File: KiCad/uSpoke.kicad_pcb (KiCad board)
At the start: 2 copper layers, 50 x 100 mm, 89 parts, among them J1 B2B-PH-K-S, J12 Amphenol 132289, J2 BAT+, J3 BAT-, J5 USB+, J6 USB-, J8 PLS-1x6, J9 PLS-1x3, Q1 AO3407A, Q2 AO3407A, Q3 AO3400, Q4 AO3400, Q5 AO3400, U2 TP4056, U4 LM3671MF-3.3, U6 STM32F103C8T6, X1 8MHz

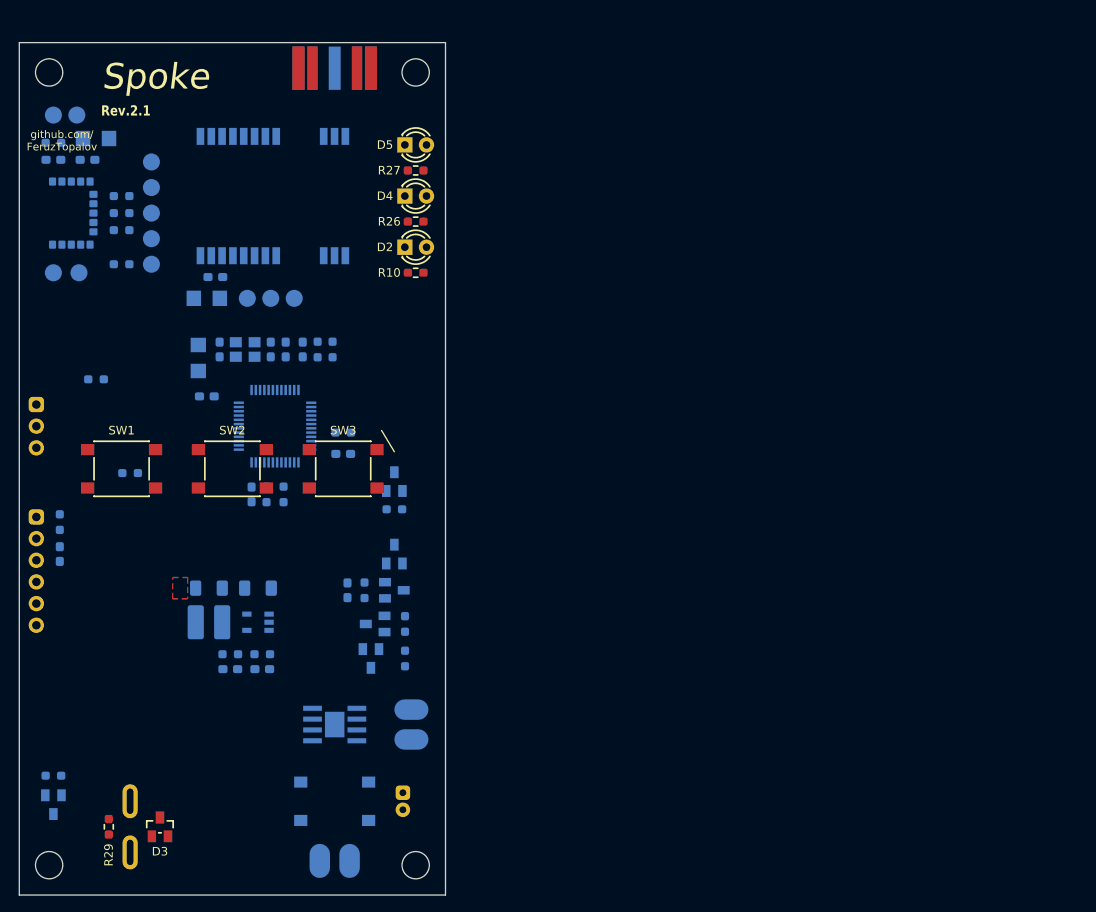
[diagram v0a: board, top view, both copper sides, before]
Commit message: Arrangement
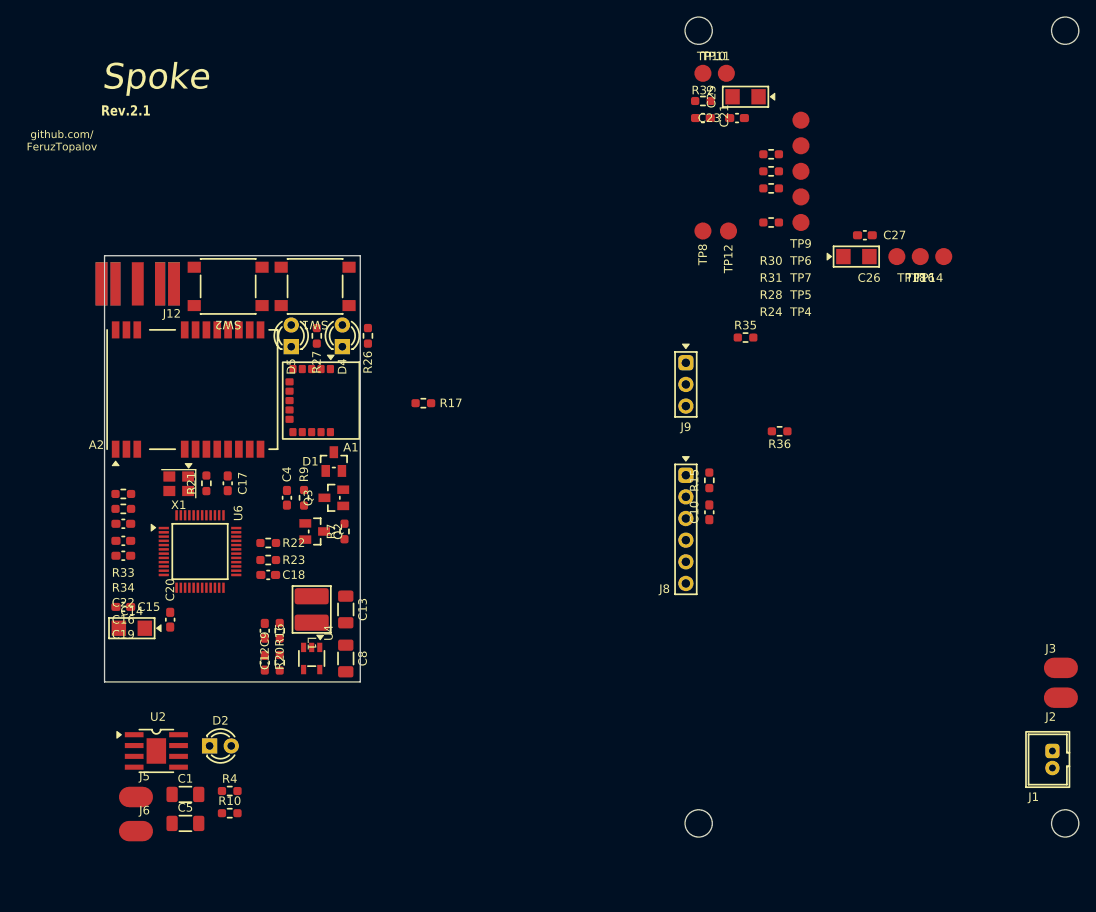
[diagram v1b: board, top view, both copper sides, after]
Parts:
- removed D3: BAT54C, Spoke:SOT-23
- removed LS1: Buzzer-Passive, Spoke:Buzzer
- removed Q1: AO3407A, Spoke:SOT-23
- removed Q4, Q5: AO3400, Spoke:SOT-23
- removed R2: 0R, Spoke:R0603
- removed R25: 300R, Spoke:R0603
- removed R29: 1kR, Spoke:R0603
- removed SW3, SW5: ~, Spoke:Button_6x6
- added C1: 10uF, Spoke:C1206, F.Cu at (94.5, 138.2)
- added C5: 10uF, Spoke:C1206, F.Cu at (94.5, 141.6)
- added R4: 3.9kR, Spoke:R0603, F.Cu at (99.7, 137.8)
- A1, A2, C10, C12, C13, C14, C15, C16, C17, C18, C19, C20, C21, C22, C23, C25, C26, C27, C4, C8, C9, D1, J1, J12, J2, J3, J5, J6, J8, J9, L1, Q2, Q3, R15, R16, R17, R20, R21, R22, R23, R24, R28, R30, R31, R32, R33, R34, R35, R36, R7, R9, TP10, TP11, TP12, TP14, TP16, TP18, TP4, TP5, TP6, TP7, TP8, TP9, U2, U4, U6, X1: moved to F.Cu
- moved C10 76.4 mm to (155.9, 105.1)
- moved C21 76.4 mm to (155.2, 58.9), turned to 0 degrees
- moved C23 76.4 mm to (159.2, 58.9), turned to 180 degrees
- moved C25 76.4 mm to (160.2, 56.4), turned to 180 degrees
- moved C26 76.4 mm to (173.2, 75.1), turned to 0 degrees
- moved C27 76.4 mm to (174.2, 72.6), turned to 0 degrees
- moved H1 76.4 mm to (154.7, 48.6)
- moved H2 76.4 mm to (197.7, 48.6)
- moved H3 76.4 mm to (154.7, 141.6)
- moved H4 76.4 mm to (197.7, 141.6)
- moved J1 76.4 mm to (196.2, 134.1)
- moved J2 76.4 mm to (197.2, 126.8), turned to 180 degrees
- moved J3 76.4 mm to (197.2, 123.3), turned to 180 degrees
- moved J8 76.4 mm to (153.2, 107.1)
- moved J9 76.4 mm to (153.2, 90.1)
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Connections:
- Q2 pad 2: Net-(Q1-S) -> +BATT
- R7 pad 1: Net-(Q1-S) -> +BATT
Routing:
- removed copper zone on F.Cu, net +3V3
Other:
- board size 50 x 100 mm -> 30 x 50 mm

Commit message: Rename to uSpoke
(cherry picked from commit a0effae12703fde22e0195c2c61b714ac3e4bfb9)

# Conflicts:
#	KiCad/uSpoke.kicad_pcb
#	KiCad/uSpoke.kicad_sch
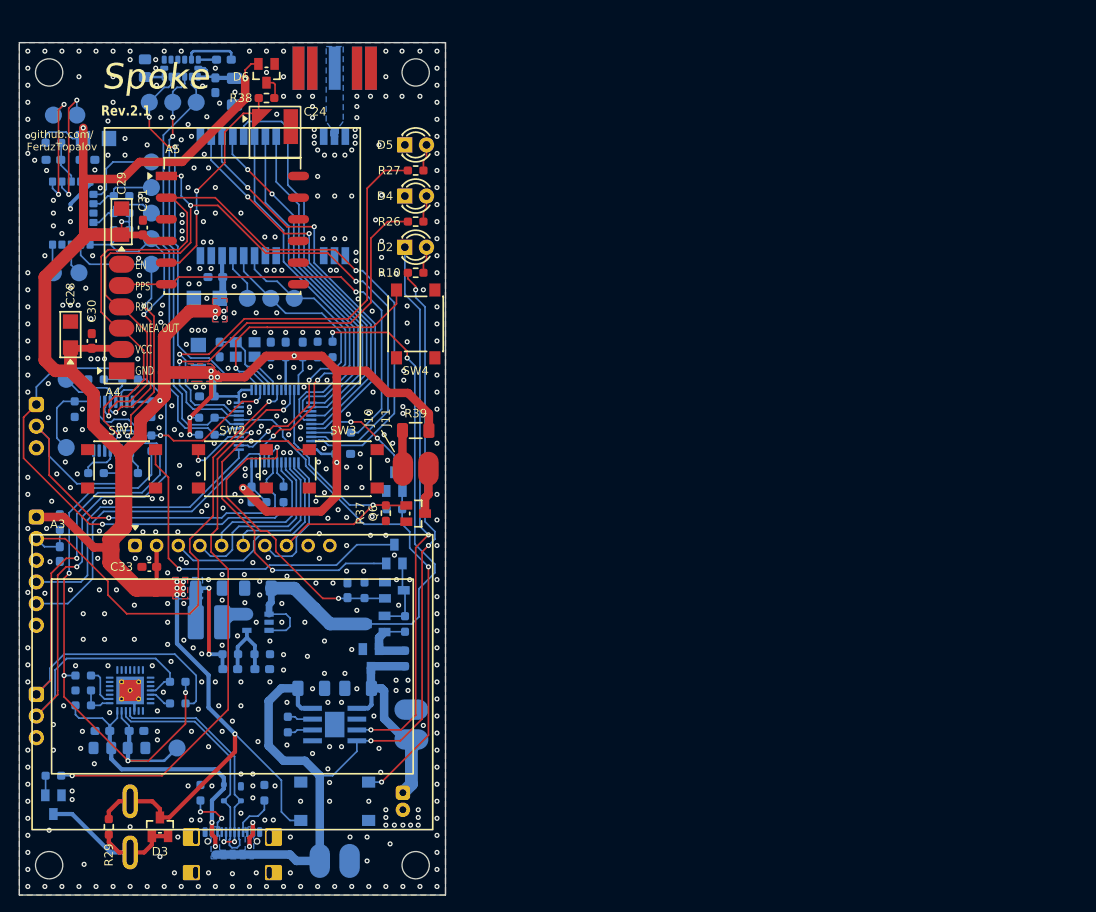
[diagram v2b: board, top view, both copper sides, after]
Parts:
- added A3: GM12864-01A, Spoke:GM12864-01A, F.Cu at (100.0, 109.0)
- added A4: G10A-F30, Spoke:G10A-F30, F.Cu at (100.0, 75.0)
- added A5: TU10-F, Spoke:TU10-F, F.Cu at (100.0, 72.0)
- added C11: 100nF, Spoke:C0603, B.Cu at (90.5, 93.0)
- added C2: 4.7uF, Spoke:C0805, B.Cu at (84.8, 132.8)
- added C24: 80 mF Supercap, Spoke:XH414HG-IV01E, F.Cu at (105.0, 60.5)
- added C28: 47uF, Spoke:C_tantA, F.Cu at (81.0, 84.2)
- added C29: 47uF, Spoke:C_tantA, F.Cu at (87.0, 71.0)
- added C3: 100nF, Spoke:C0603, B.Cu at (84.8, 130.8)
- added C30: 100nF, Spoke:C0603, F.Cu at (83.5, 85.0)
- added C31: 100nF, Spoke:C0603, F.Cu at (89.5, 71.7)
- added C32: 4.7uF, Spoke:C0805, B.Cu at (89.8, 53.0)
- added C33: 100nF, Spoke:C0603, F.Cu at (90.2, 111.5)
- added C34: 10uF, Spoke:C1206, B.Cu at (100.2, 55.8)
- added C35: 100nF, Spoke:C0603, B.Cu at (98.0, 55.0)
- added C36: 220nF, Spoke:C0603, B.Cu at (99.0, 52.0)
- added C6: 100nF, Spoke:C0603, B.Cu at (88.8, 130.8)
- added C7: 4.7uF, Spoke:C0805, B.Cu at (88.8, 132.8)
- added D3: BAT54C, Spoke:SOT-23, F.Cu at (91.5, 142.0)
- added D6: BAT54C, Spoke:SOT-23, F.Cu at (104.0, 53.6)
- added J10: BL-A, Spoke:Pad_oval, F.Cu at (120.0, 100.0)
- added J11: BL-C, Spoke:Pad_oval, F.Cu at (123.0, 100.0)
- added J4: GCT USB4105/USB4110, Spoke:USB_C_16p_GCT4105, B.Cu at (100.0, 146.3)
- added J7: PLS-1x3, Spoke:Header_1x3, B.Cu at (77.0, 129.0)
- added LS1: Buzzer-Passive, Spoke:Buzzer, B.Cu at (88.0, 142.0)
- added Q1: AO3407A, Spoke:SOT-23, B.Cu at (116.2, 122.2)
- added Q4: AO3400, Spoke:SOT-23, B.Cu at (119.0, 101.5)
- added Q5: AO3400, Spoke:SOT-23, B.Cu at (79.0, 139.4)
- added Q6: AO3400, Spoke:SOT-23, F.Cu at (121.5, 105.2)
- added R1: 5.1kR, Spoke:R0603, B.Cu at (96.2, 138.0)
- added R11: 100kR, Spoke:R0603, B.Cu at (93.6, 125.0)
- added R12: 1kR, Spoke:R0603, B.Cu at (93.6, 127.5)
- added R13: 100kR, Spoke:R0603, B.Cu at (90.5, 97.0)
- added R14: 100kR, Spoke:R0603, B.Cu at (81.5, 93.0)
- added R18: 0R, Spoke:R0603, B.Cu at (88.0, 89.5)
- added R19: 0R, Spoke:R0603, B.Cu at (84.0, 100.5)
- added R2: 0R, Spoke:R0603, B.Cu at (120.2, 122.2)
- added R25: 300R, Spoke:R0603, B.Cu at (79.0, 136.0)
- added R29: 1kR, Spoke:R0603, F.Cu at (85.5, 142.0)
- added R3: 5.1kR, Spoke:R0603, B.Cu at (103.8, 138.0)
- added R37: 100kR, Spoke:R0603, F.Cu at (118.0, 105.2)
- added R38: 300R, Spoke:R0603, F.Cu at (104.0, 56.5)
- added R39: 100R, Spoke:R1206, F.Cu at (121.5, 95.5)
- added R40: 3.9kR, Spoke:R0603, B.Cu at (97.0, 96.0)
- added R41: 3.9kR, Spoke:R0603, B.Cu at (97.0, 94.0)
- added R5: 22.1kR, Spoke:R0603, B.Cu at (82.5, 127.8)
- added R6: 47.5kR, Spoke:R0603, B.Cu at (82.5, 126.0)
- added R8: 1kR, Spoke:R0603, B.Cu at (82.5, 124.2)
- added SW3: ~, Spoke:Button_6x6, F.Cu at (113.0, 100.0)
- added SW4: ~, Spoke:Button_6x6, F.Cu at (121.5, 83.0)
- added SW5: ~, Spoke:Button_6x6, B.Cu at (112.0, 139.0)
- added TP1: Pad-Round, Spoke:Pad_round, B.Cu at (93.5, 132.8)
- added TP13: Pad-Round, Spoke:Pad_round, B.Cu at (95.8, 57.0)
- added TP15: Pad-Round, Spoke:Pad_round, B.Cu at (93.0, 57.0)
- added TP17: Pad-Round, Spoke:Pad_round, B.Cu at (90.2, 57.0)
- added TP2: Pad-Round, Spoke:Pad_round, B.Cu at (80.5, 89.5)
- added TP3: Pad-Round, Spoke:Pad_round, B.Cu at (80.5, 97.5)
- added U1: SP0503BAHTG, Spoke:SOT-143, B.Cu at (100.0, 138.0)
- added U3: CP2102N-A02-GQFN28, Spoke:QFN-28, B.Cu at (88.0, 126.0)
- added U5: 74HC4052PW, Spoke:TSSOP-16, B.Cu at (86.0, 95.0)
- added U7: LSM303DLHC, Spoke:LGA-14, B.Cu at (94.0, 53.0)
- A1, A2, C1, C10, C12, C13, C14, C15, C16, C17, C18, C19, C20, C21, C22, C23, C25, C26, C27, C4, C5, C8, C9, D1, J1, J12, J2, J3, J5, J6, J8, J9, L1, Q2, Q3, R15, R16, R17, R20, R21, R22, R23, R24, R28, R30, R31, R32, R33, R34, R35, R36, R4, R7, R9, TP10, TP11, TP12, TP14, TP16, TP18, TP4, TP5, TP6, TP7, TP8, TP9, U2, U4, U6, X1: moved to B.Cu
- moved C10 76.4 mm to (79.8, 110.0)
- moved C21 76.4 mm to (79.0, 63.8), turned to 180 degrees
- moved C23 76.4 mm to (83.0, 63.8), turned to 0 degrees
- moved C25 76.4 mm to (84.0, 61.2), turned to 0 degrees
- moved C26 76.4 mm to (97.0, 80.0), turned to 180 degrees
- moved C27 76.4 mm to (98.0, 77.5), turned to 180 degrees
- moved H1 76.4 mm to (78.5, 53.5)
- moved H2 76.4 mm to (121.5, 53.5)
- moved H3 76.4 mm to (78.5, 146.5)
- moved H4 76.4 mm to (121.5, 146.5)
- moved J1 76.4 mm to (120.0, 139.0)
- moved J2 76.4 mm to (121.0, 131.8), turned to 0 degrees
- moved J3 76.4 mm to (121.0, 128.2), turned to 0 degrees
- moved J8 76.4 mm to (77.0, 112.0)
- moved J9 76.4 mm to (77.0, 95.0)
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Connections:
- J8 pad 3: BOOT0 -> GND
- Q2 pad 2: +BATT -> Net-(Q1-S)
- R7 pad 1: +BATT -> Net-(Q1-S)
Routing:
- net +3V3: track 0.00 -> 371.2 mm, vias 0 -> 25
- net VBUS: track 0.00 -> 154.2 mm, vias 0 -> 7
- net GPS_TXD: track 0.00 -> 102.7 mm, vias 0 -> 2
- net GPS_RXD: track 0.00 -> 97.2 mm, vias 0 -> 4
- net USB_RXD: track 0.00 -> 80.4 mm, vias 0 -> 1
- net USB_TXD: track 0.00 -> 79.2 mm, vias 0 -> 1
- net VDD: track 0.00 -> 74.2 mm, vias 0 -> 4
- net VCC: track 0.00 -> 72.9 mm, vias 0 -> 2
- net BUZZER: track 0.00 -> 66.1 mm, vias 0 -> 2
- net BOOT0: track 0.00 -> 64.3 mm, vias 0 -> 2
- net Net-(D2-K): track 0.00 -> 64.3 mm, vias 0 -> 2
- net CONSOLE_RXD: track 0.00 -> 61.4 mm, vias 0 -> 1
- net CONSOLE_TXD: track 0.00 -> 61.4 mm, vias 0 -> 1
- net MCU_RESET: track 0.00 -> 59.4 mm, vias 0 -> 1
- net LED_GREEN: track 0.00 -> 55.5 mm, vias 0 -> 1
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- added copper zone on B.Cu, net +3V3
- added copper zone on F.Cu, net +3V3
- added copper zone on B.Cu, net /ANT
- added copper zone on B.Cu, net GND
- added copper zone on F.Cu, net GND
- added copper zone on B.Cu, net VBUS
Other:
- board size 30 x 50 mm -> 50 x 100 mm
